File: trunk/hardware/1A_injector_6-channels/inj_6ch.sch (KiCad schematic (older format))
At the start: 35 parts, among them P1 HEADER_10X2, P2 CONN_2, P3 CONN_3, P4 CONN_2, P5 CONN_3, P7 HEADER_10X2, Q1 OVP_DRIVER, Q2 OVP_DRIVER, Q3 OVP_DRIVER, Q4 OVP_DRIVER, Q5 OVP_DRIVER, Q6 OVP_DRIVER

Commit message: working with BOM
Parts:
- R1, R13, R14, R15, R16, R17, R18: mfg,mfg# VISHAY,CRCW0805100KFKEA -> Panasonic,ERJ-6GEYJ102V; vend1,vend1# digi,CRCW0805100KFKEA -> digi,P1.0KACT-ND
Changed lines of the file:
@@
 F 2 "SM0805" V 1130 600 60  0001 C CNN
 F 3 "" H 4200 2625 60  0001 C CNN
-F 4 "VISHAY,CRCW0805100KFKEA" V 1130 600 60  0001 C CNN "mfg,mfg#"
-F 5 "digi,CRCW0805100KFKEA" V 1130 600 60  0001 C CNN "vend1,vend1#"
+F 4 "Panasonic,ERJ-6GEYJ102V" V 1130 600 60  0001 C CNN "mfg,mfg#"
+F 5 "digi,P1.0KACT-ND" V 1130 600 60  0001 C CNN "vend1,vend1#"
 	1    4200 2625
 	0    1    -1   0
@@
 F 2 "SM0805" V 1130 -100 60  0001 C CNN
 F 3 "" H 4200 2275 60  0001 C CNN
-F 4 "VISHAY,CRCW0805100KFKEA" V 1130 -100 60  0001 C CNN "mfg,mfg#"
-F 5 "digi,CRCW0805100KFKEA" V 1130 -100 60  0001 C CNN "vend1,vend1#"
+F 4 "Panasonic,ERJ-6GEYJ102V" V 1130 -100 60  0001 C CNN "mfg,mfg#"
+F 5 "digi,P1.0KACT-ND" V 1130 -100 60  0001 C CNN "vend1,vend1#"
 	1    4200 2275
 	0    1    1    0
@@
 F 2 "SM0805" V 1130 3100 60  0001 C CNN
 F 3 "" H 4200 3875 60  0001 C CNN
-F 4 "VISHAY,CRCW0805100KFKEA" V 1130 3100 60  0001 C CNN "mfg,mfg#"
-F 5 "digi,CRCW0805100KFKEA" V 1130 3100 60  0001 C CNN "vend1,vend1#"
+F 4 "Panasonic,ERJ-6GEYJ102V" V 1130 3100 60  0001 C CNN "mfg,mfg#"
+F 5 "digi,P1.0KACT-ND" V 1130 3100 60  0001 C CNN "vend1,vend1#"
 	1    4200 3875
 	0    1    -1   0
@@
 F 2 "SM0805" V 1130 2400 60  0001 C CNN
 F 3 "" H 4200 3525 60  0001 C CNN
-F 4 "VISHAY,CRCW0805100KFKEA" V 1130 2400 60  0001 C CNN "mfg,mfg#"
-F 5 "digi,CRCW0805100KFKEA" V 1130 2400 60  0001 C CNN "vend1,vend1#"
+F 4 "Panasonic,ERJ-6GEYJ102V" V 1130 2400 60  0001 C CNN "mfg,mfg#"
+F 5 "digi,P1.0KACT-ND" V 1130 2400 60  0001 C CNN "vend1,vend1#"
 	1    4200 3525
 	0    1    1    0
@@
 F 2 "SM0805" V 1130 4900 60  0001 C CNN
 F 3 "" H 4200 4775 60  0001 C CNN
-F 4 "VISHAY,CRCW0805100KFKEA" V 1130 4900 60  0001 C CNN "mfg,mfg#"
-F 5 "digi,CRCW0805100KFKEA" V 1130 4900 60  0001 C CNN "vend1,vend1#"
+F 4 "Panasonic,ERJ-6GEYJ102V" V 1130 4900 60  0001 C CNN "mfg,mfg#"
+F 5 "digi,P1.0KACT-ND" V 1130 4900 60  0001 C CNN "vend1,vend1#"
 	1    4200 4775
 	0    1    1    0
@@
 F 2 "SM0805" V 1130 5600 60  0001 C CNN
 F 3 "" H 4200 5125 60  0001 C CNN
-F 4 "VISHAY,CRCW0805100KFKEA" V 1130 5600 60  0001 C CNN "mfg,mfg#"
-F 5 "digi,CRCW0805100KFKEA" V 1130 5600 60  0001 C CNN "vend1,vend1#"
+F 4 "Panasonic,ERJ-6GEYJ102V" V 1130 5600 60  0001 C CNN "mfg,mfg#"
+F 5 "digi,P1.0KACT-ND" V 1130 5600 60  0001 C CNN "vend1,vend1#"
 	1    4200 5125
 	0    1    -1   0
@@
 F 2 "SM0805" V 2080 4100 60  0001 C CNN
 F 3 "" H 5150 6475 60  0001 C CNN
-F 4 "VISHAY,CRCW0805100KFKEA" V 2080 4100 60  0001 C CNN "mfg,mfg#"
-F 5 "digi,CRCW0805100KFKEA" V 2080 4100 60  0001 C CNN "vend1,vend1#"
+F 4 "Panasonic,ERJ-6GEYJ102V" V 2080 4100 60  0001 C CNN "mfg,mfg#"
+F 5 "digi,P1.0KACT-ND" V 2080 4100 60  0001 C CNN "vend1,vend1#"
 	1    5150 6475
 	0    -1   1    0

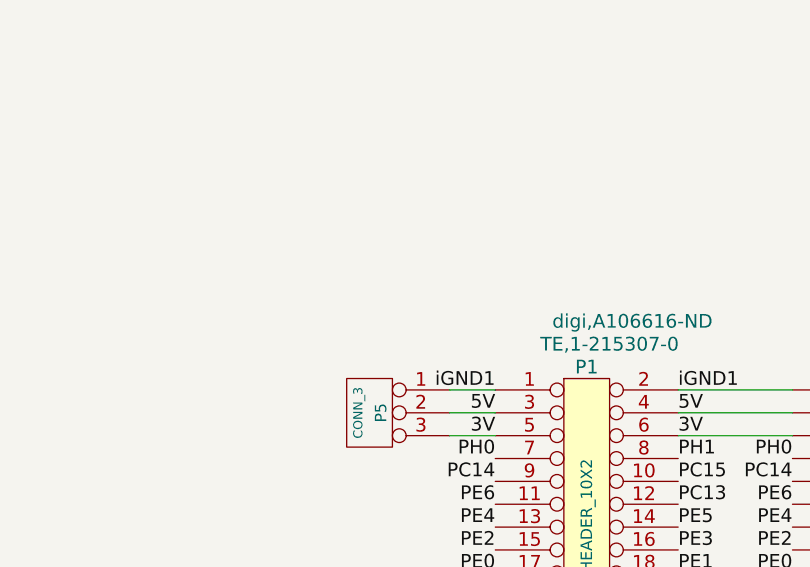
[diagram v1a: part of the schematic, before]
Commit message: BOM improvements
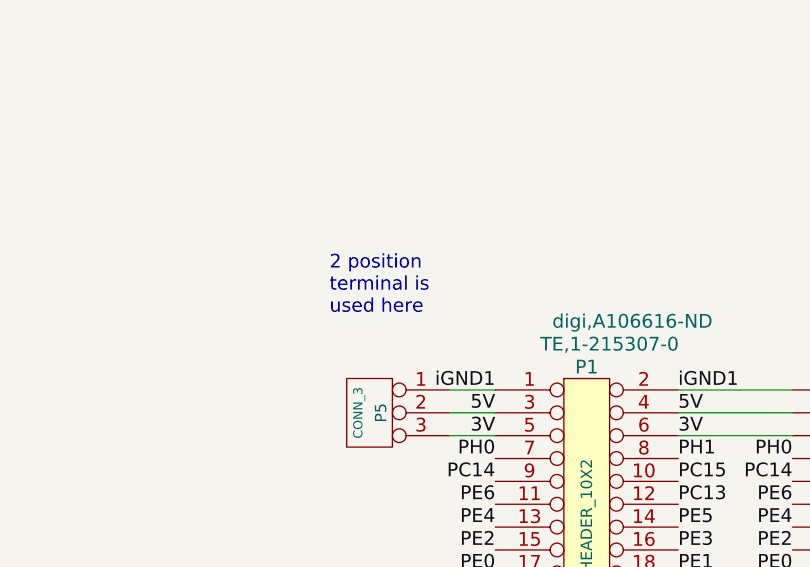
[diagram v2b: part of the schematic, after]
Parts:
- P2, P4: mfg 1760490000 -> (none); mfg,mfg# (none) -> OST,OSTTC022162; vend1,vend1# (none) -> digi,ED2609-ND
- P3: mfg# 1760500000 -> (none); mfg,mfg# (none) -> OST,OSTTC032162; vend1,vend1# (none) -> digi,ED2610-ND
- P5: mfg# 1760500000 -> (none); mfg,mfg# (none) -> OST,OSTTC022162; vend1,vend1# (none) -> digi,ED2609-ND
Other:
- note added: "2 position\nterminal is\nused here"
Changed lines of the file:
@@
 Sheet 1 1
 Title "6 Channel Injector"
-Date "24 dec 2013"
+Date "30 dec 2013"
 Rev "A-6"
 Comp "http://code.google.com/p/daecu/"
@@
 F 2 "bornier3" H 5800 3625 60  0001 C CNN
 F 3 "" H 5800 3625 60  0000 C CNN
-F 4 "1760500000" V 5800 3625 60  0001 C CNN "mfg#"
+F 4 "OST,OSTTC032162" V 5800 3625 60  0001 C CNN "mfg,mfg#"
+F 5 "digi,ED2610-ND" V 5800 3625 60  0001 C CNN "vend1,vend1#"
 	1    5800 3625
 	1    0    0    1
@@
 F 2 "bornier2" H 5800 3925 60  0001 C CNN
 F 3 "" H 5800 3925 60  0000 C CNN
-F 4 "1760490000" V 5800 3925 60  0001 C CNN "mfg"
+F 4 "OST,OSTTC022162" V 5800 3925 60  0001 C CNN "mfg,mfg#"
+F 5 "digi,ED2609-ND" V 5800 3925 60  0001 C CNN "vend1,vend1#"
 	1    5800 3925
 	1    0    0    1
@@
 F 2 "bornier2" H 5800 3325 60  0001 C CNN
 F 3 "" H 5800 3325 60  0000 C CNN
-F 4 "1760490000" V 5800 3325 60  0001 C CNN "mfg"
+F 4 "OST,OSTTC022162" V 5800 3325 60  0001 C CNN "mfg,mfg#"
+F 5 "digi,ED2609-ND" V 5800 3325 60  0001 C CNN "vend1,vend1#"
 	1    5800 3325
 	1    0    0    1
@@
 F 2 "bornier3" H 725 6475 60  0001 C CNN
 F 3 "" H 725 6475 60  0000 C CNN
-F 4 "1760500000" V 725 6475 60  0001 C CNN "mfg#"
+F 4 "OST,OSTTC022162" V 725 6475 60  0001 C CNN "mfg,mfg#"
+F 5 "digi,ED2609-ND" V 725 6475 60  0001 C CNN "vend1,vend1#"
 	1    725  6475
 	-1   0    0    -1
@@
 	1    0    0    -1
 $EndComp
+Text Notes 550  6050 0    60   ~ 0
+2 position\nterminal is\nused here
 $EndSCHEMATC
